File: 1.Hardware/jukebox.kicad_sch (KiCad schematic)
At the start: 34 parts, among them J1 USB_C_Receptacle_USB2.0_16P, Q1 SS8050, Q2 SS8050, SW1 SW_Push, SW2 SW_Push, U1 CP2102N-Axx-xQFN28, U4 AMS1117-3.3

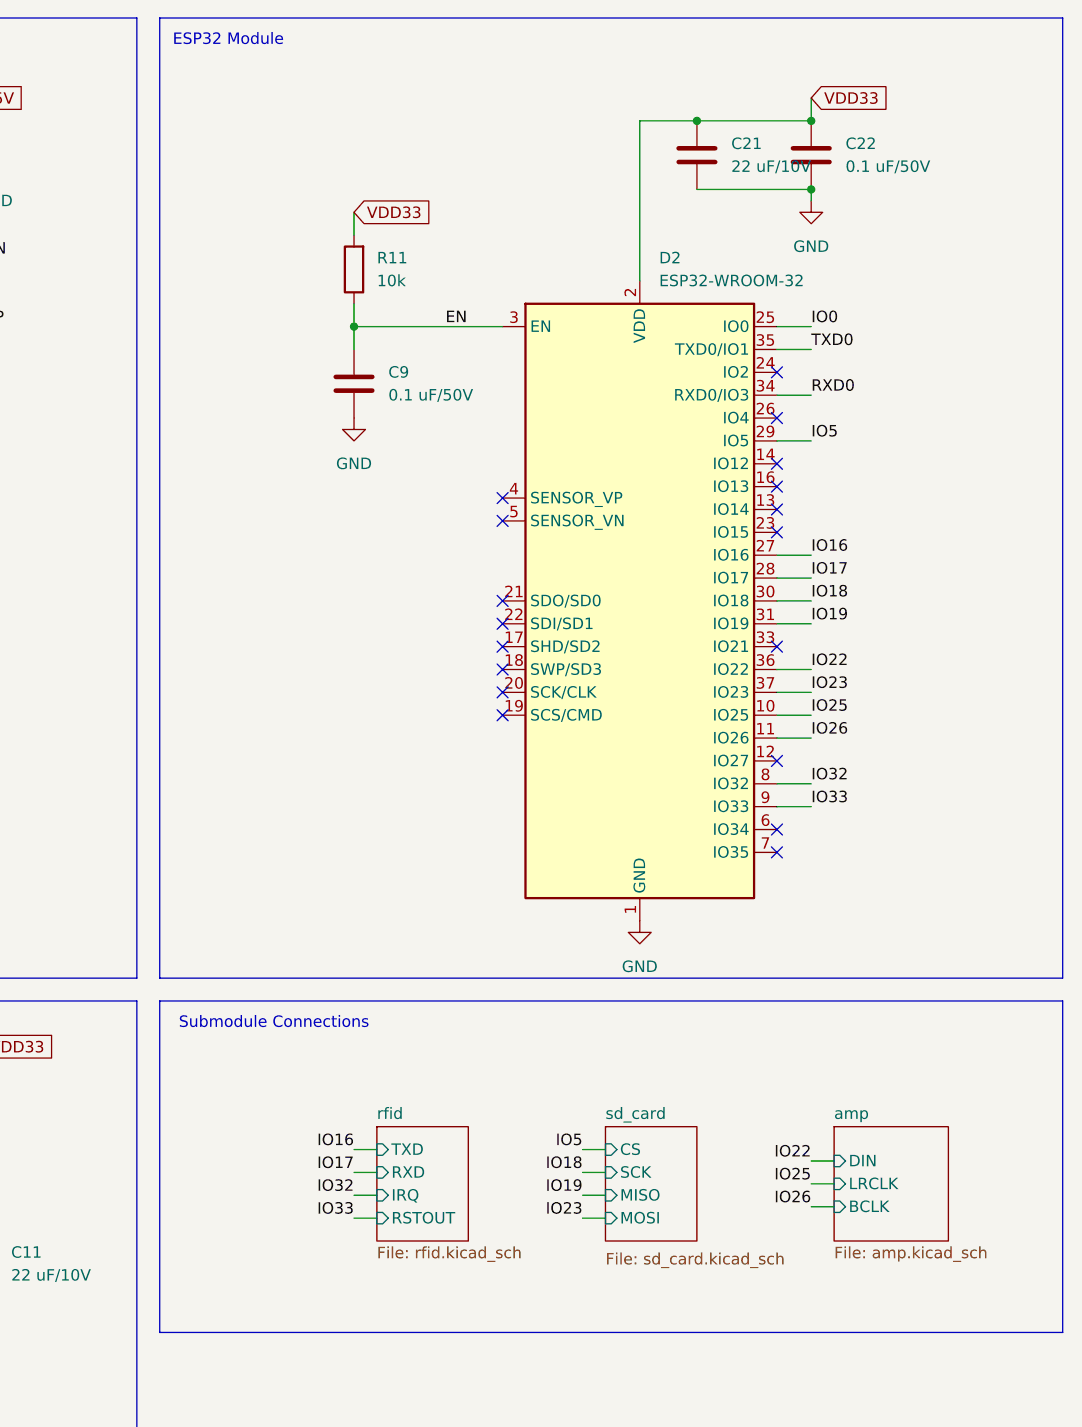
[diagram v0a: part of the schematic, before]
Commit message: ready for routing/placement
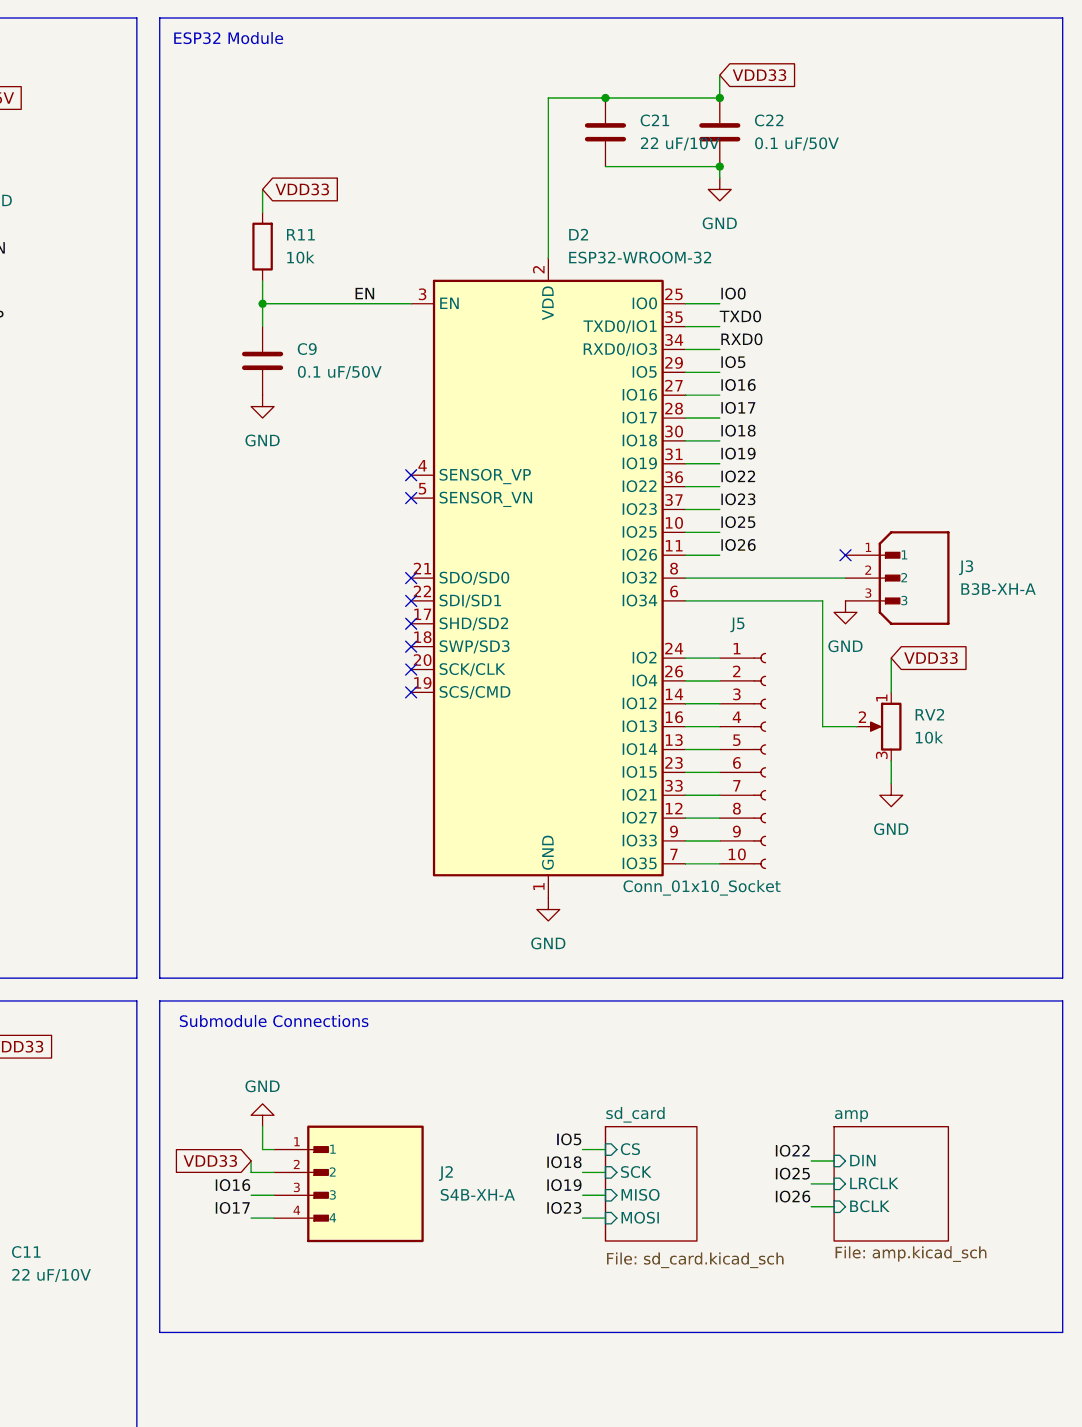
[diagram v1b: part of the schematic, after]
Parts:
- added J2: S4B-XH-A, S4B-XH-A:JST_S4B-XH-A, symbol S4B-XH-A:S4B-XH-A
- added J3: B3B-XH-A, B3B_XH_A:JST_B3B-XH-A, symbol B3B-XH-A:B3B-XH-A
- added J5: Conn_01x10_Socket, Connector_PinHeader_2.54mm:PinHeader_1x10_P2.54mm_Vertical, symbol Connector:Conn_01x10_Socket
- added RV2: 10k, 3306K:TRIM_3306K-1-202, symbol Device:R_Potentiometer
- C10, C11, C21: footprint Capacitor_SMD:C_0603_1608Metric -> Capacitor_SMD:C_0603_1608Metric_Pad1.08x0.95mm_HandSolder
- C14, C15, C19, C20, C22, C9: footprint Capacitor_SMD:C_0402_1005Metric -> Capacitor_SMD:C_0603_1608Metric_Pad1.08x0.95mm_HandSolder
- D1: footprint LED_SMD:LED_0603_1608Metric -> LED_SMD:LED_0603_1608Metric_Pad1.05x0.95mm_HandSolder
- R11, R17, R18, R21, R22, R23, R24, R25, R26, R7: footprint Resistor_SMD:R_0402_1005Metric -> Resistor_SMD:R_0603_1608Metric_Pad0.98x0.95mm_HandSolder
- R12, R8: footprint (none) -> Resistor_SMD:R_0603_1608Metric_Pad0.98x0.95mm_HandSolder
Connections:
- net GND: now also J2.1, J3.3, RV2.3
- net IO16: now also J2.3
- net IO17: now also J2.4
- net VDD33: now also J2.2, RV2.1
- net at D2.12 (IO27): now also J5.8 (Pin_8)
- net at D2.13 (IO14): now also J5.5 (Pin_5)
- net at D2.14 (IO12): now also J5.3 (Pin_3)
- net at D2.16 (IO13): now also J5.4 (Pin_4)
- net at D2.23 (IO15): now also J5.6 (Pin_6)
- net at D2.24 (IO2): now also J5.1 (Pin_1)
- net at D2.26 (IO4): now also J5.2 (Pin_2)
- net at D2.33 (IO21): now also J5.7 (Pin_7)
- net at D2.6 (IO34): now also RV2.2
- net at D2.7 (IO35): now also J5.10 (Pin_10)
- net IO32: no longer names the net of D2.8 (IO32)
- net IO32: now also J3.2
- net IO33: no longer names the net of D2.9 (IO33)
- net IO33: now also J5.9 (Pin_9)
- no-connect marks 35 -> 26
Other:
- removed sheet rfid
- moved on the sheet: C21, C22, C9, D2, R11
